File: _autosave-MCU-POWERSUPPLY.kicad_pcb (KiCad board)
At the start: 2 copper layers, 9 parts, among them J3 Barrel_Jack, J4 USB_B_Micro, U4 LM2596S-5

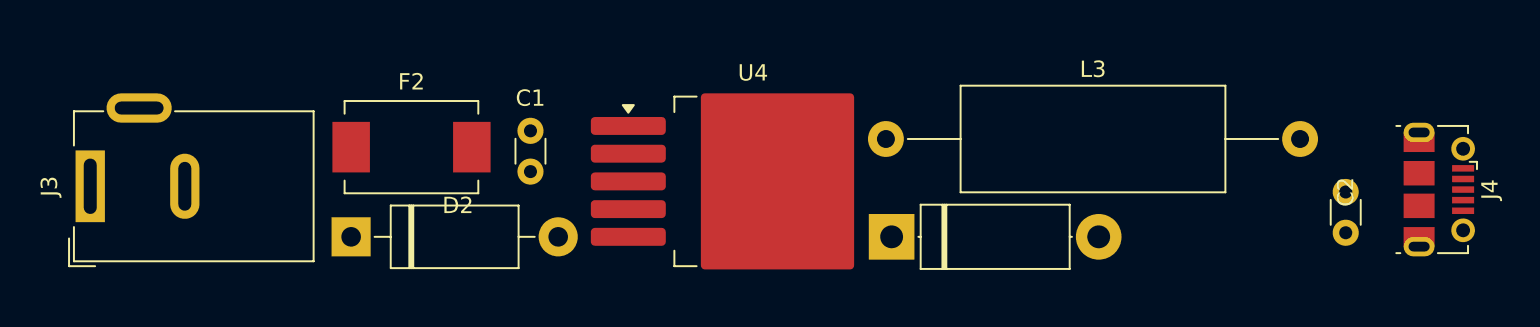
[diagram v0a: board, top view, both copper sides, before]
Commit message: a
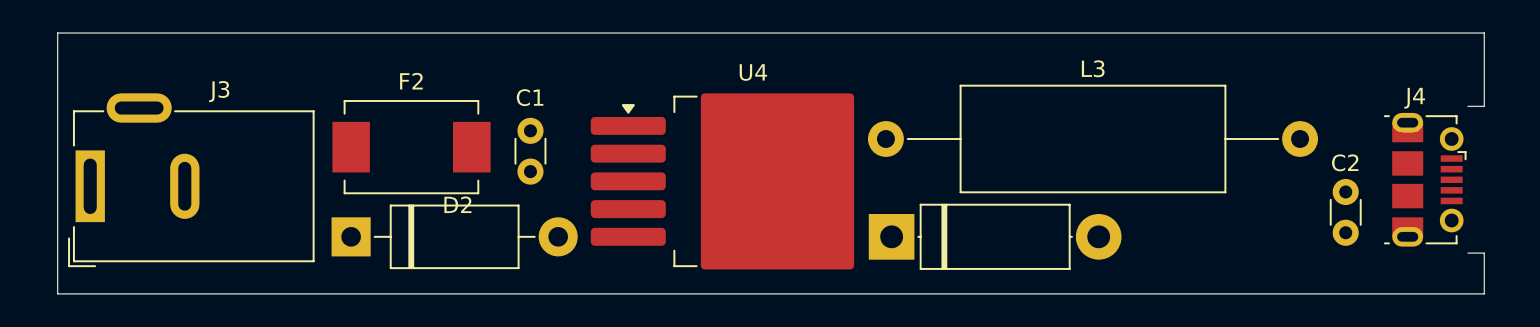
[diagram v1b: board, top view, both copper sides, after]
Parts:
- moved J4 0.92 mm to (181.0, 109.5)
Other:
- board outline added: 87.5 x 16 mm
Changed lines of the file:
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@@
 		(tags "connector barrel jack")
 		(property "Reference" "J3"
-			(at 0 -2.5 90)
+			(at 5.9 8 180)
 			(layer "F.SilkS")
 			(effects
@@
 		(tags "C Disc series Radial pin pitch 2.50mm diameter 3.0mm width 1.6mm Capacitor")
 		(property "Reference" "C2"
-			(at 0 0 90)
+			(at -1.75 0 180)
 			(layer "F.SilkS")
 			(effects
@@
 	(footprint "Connector_USB:USB_Micro-B_Molex-105017-0001"
 		(layer "F.Cu")
-		(at 181.7375 110.1 -90)
+		(at 181.0375 109.5 -90)
 		(descr "http://www.molex.com/pdm_docs/sd/1050170001_sd.pdf")
 		(tags "Micro-USB SMD Typ-B")
 		(property "Reference" "J4"
-			(at 0 -3.1125 90)
+			(at -5.1 0.7375 0)
 			(layer "F.SilkS")
 			(effects
@@
 			)
 			(layer "F.Fab")
-		)
-		(fp_text user "${REFERENCE}"
-			(at 0 0.8875 90)
-			(layer "F.Fab")
-			(effects
-				(font
-					(size 1 1)
-					(thickness 0.15)
-				)
-			)
 		)
 		(pad "1" smd rect
@@
 		)
 	)
+	(gr_line
+		(start 184.5 114)
+		(end 184.5 116.5)
+		(stroke
+			(width 0.05)
+			(type default)
+		)
+		(layer "Edge.Cuts")
+	)
+	(gr_line
+		(start 184.5 116.5)
+		(end 97 116.5)
+		(stroke
+			(width 0.05)
+			(type default)
+		)
+		(layer "Edge.Cuts")
+	)
+	(gr_line
+		(start 97 100.5)
+		(end 97 116.5)
+		(stroke
+			(width 0.05)
+			(type default)
+		)
+		(layer "Edge.Cuts")
+	)
+	(gr_line
+		(start 184.5 114)
+		(end 183.5 114)
+		(stroke
+			(width 0.05)
+			(type default)
+		)
+		(layer "Edge.Cuts")
+	)
+	(gr_line
+		(start 184.5 100.5)
+		(end 184.5 105)
+		(stroke
+			(width 0.05)
+			(type default)
+		)
+		(layer "Edge.Cuts")
+	)
+	(gr_line
+		(start 97 100.5)
+		(end 184.5 100.5)
+		(stroke
+			(width 0.05)
+			(type default)
+		)
+		(layer "Edge.Cuts")
+	)
+	(gr_line
+		(start 184.5 105)
+		(end 183.5 105)
+		(stroke
+			(width 0.05)
+			(type default)
+		)
+		(layer "Edge.Cuts")
+	)
 	(embedded_fonts no)
